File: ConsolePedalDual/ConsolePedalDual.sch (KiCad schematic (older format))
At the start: 20 parts, among them J1 AudioJack3, J2 AudioJack2, J3 Conn_02x25_Odd_Even, J4 Conn_02x25_Odd_Even, SW1 Bypass

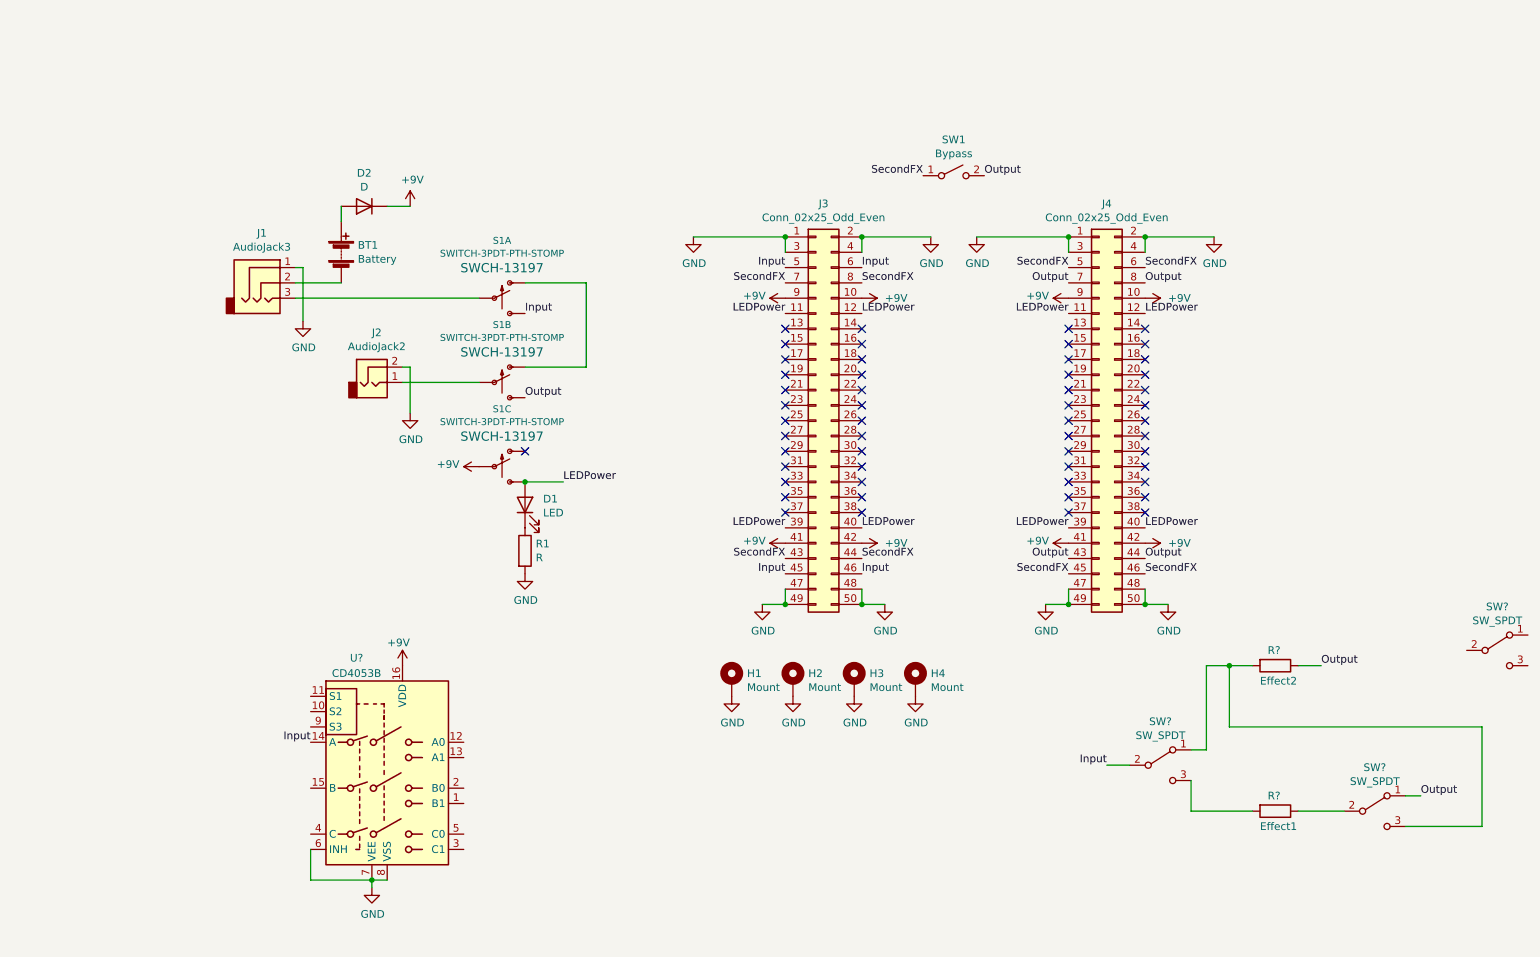
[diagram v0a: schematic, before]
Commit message: Finished schematic. Trying to figure out how to fit all these components on this board
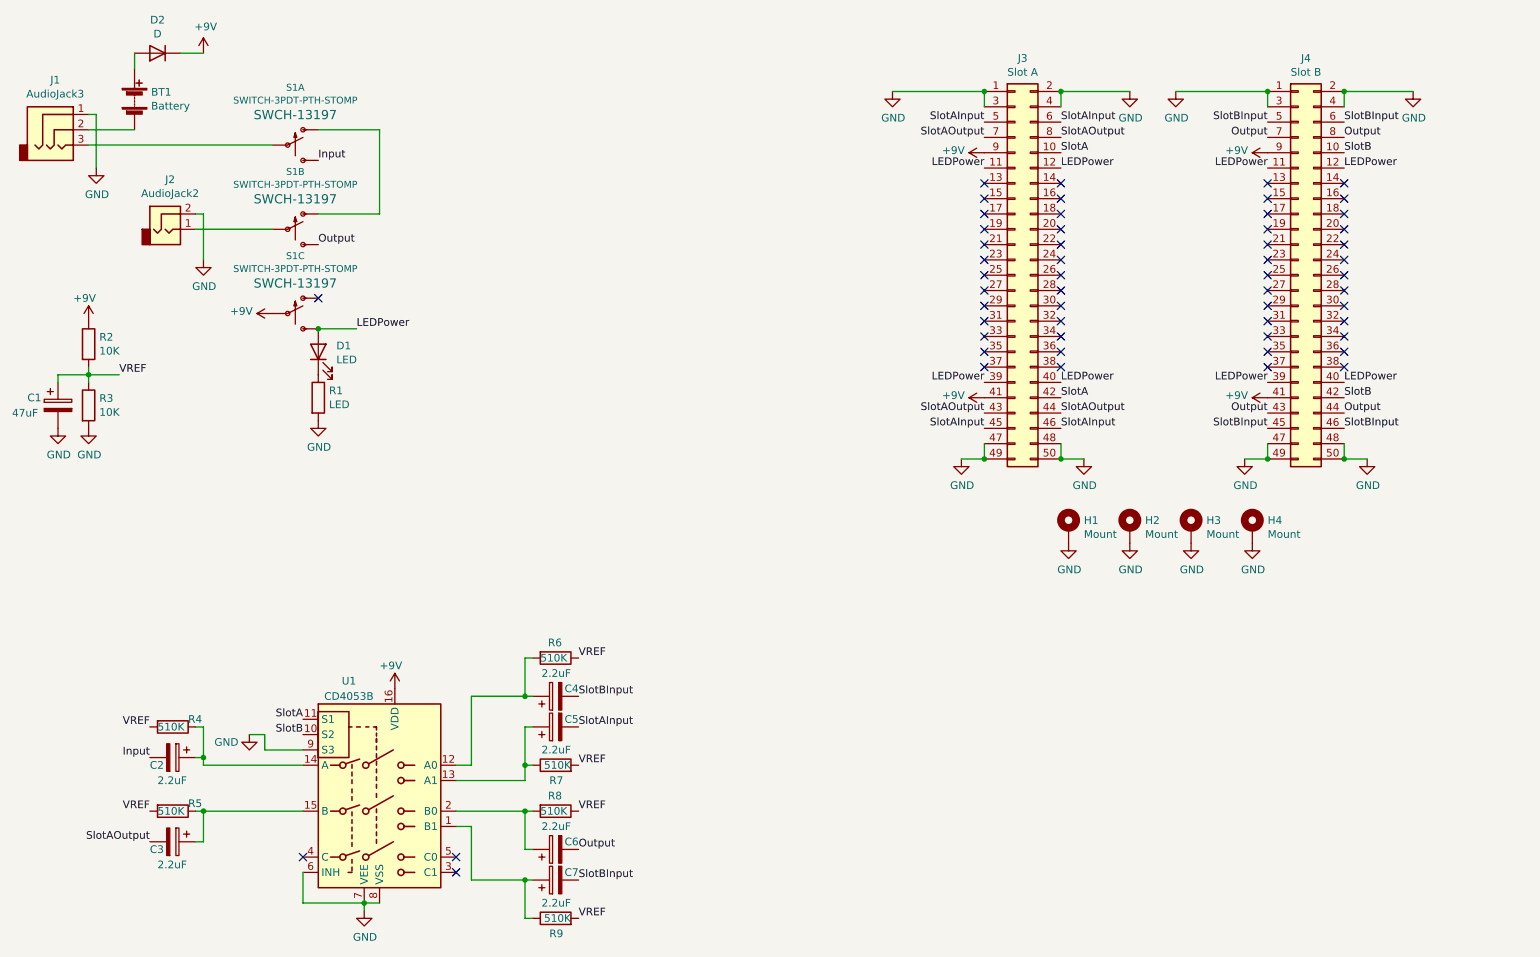
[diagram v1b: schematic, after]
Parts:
- removed R?: Effect1, Resistor_THT:R_Axial_DIN0207_L6.3mm_D2.5mm_P10.16mm_Horizontal, symbol Device:R
- removed R?: Effect2, Resistor_THT:R_Axial_DIN0207_L6.3mm_D2.5mm_P10.16mm_Horizontal, symbol Device:R
- removed SW1: Bypass, Connector_PinSocket_2.54mm:PinSocket_1x02_P2.54mm_Vertical, symbol Switch:SW_SPST
- removed SW? (x3): SW_SPDT, symbol Switch:SW_SPDT
- added C1: 47uF, Capacitor_THT:CP_Radial_D6.3mm_P2.50mm, symbol Device:CP
- added C2, C3, C4, C5, C6, C7: 2.2uF, Capacitor_THT:CP_Radial_D4.0mm_P2.00mm, symbol Device:CP
- added R2, R3: 10K, Resistor_THT:R_Axial_DIN0207_L6.3mm_D2.5mm_P10.16mm_Horizontal, symbol Device:R
- added R4, R5, R6, R7, R8, R9: 510K, Resistor_THT:R_Axial_DIN0207_L6.3mm_D2.5mm_P10.16mm_Horizontal, symbol Device:R
- J3: value Conn_02x25_Odd_Even -> Slot A
- J4: value Conn_02x25_Odd_Even -> Slot B
- R1: value R -> LED
- U1: renamed from U?; footprint (none) -> Package_DIP:DIP-16_W7.62mm_Socket
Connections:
- net +9V: now also R2.1; no longer J3.10 (Pin_10), J3.42 (Pin_42), J4.10 (Pin_10), J4.42 (Pin_42)
- net GND: now also U1.9 (S3), C1.2, R3.2
- net Input: now also C2.2; no longer J3.45 (Pin_45), J3.46 (Pin_46), J3.5 (Pin_5), J3.6 (Pin_6), U1.14 (A)
- net Output: now also C6.2
- net at U1.1 (B1): now also C7.1, R9.1
- net SlotB: now reaches U1.10 (S2)
- net SlotB: now also J4.10 (Pin_10), J4.42 (Pin_42)
- net SlotA: now reaches U1.11 (S1)
- net SlotA: now also J3.10 (Pin_10), J3.42 (Pin_42)
- net at U1.12 (A0): now also C4.1, R6.2
- net at U1.13 (A1): now also C5.1, R7.1
- net at U1.15 (B): now also C3.1, R5.1
- net at U1.2 (B0): now also C6.1, R8.2
- net SecondFX renamed SlotAOutput
- net SlotAOutput: now also C3.2; no longer J4.45 (Pin_45), J4.46 (Pin_46), J4.5 (Pin_5), J4.6 (Pin_6)
- new net: C2.1, R4.1, U1.14 (A)
- new net SlotAInput: C5.2, J3.45 (Pin_45), J3.46 (Pin_46), J3.5 (Pin_5), J3.6 (Pin_6)
- new net SlotBInput: C4.2, C7.2, J4.45 (Pin_45), J4.46 (Pin_46), J4.5 (Pin_5), J4.6 (Pin_6)
- new net VREF: C1.1, R2.2, R3.1, R4.2, R5.2, R6.1, R7.2, R8.1, R9.2
- no-connect marks 53 -> 56
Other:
- moved on the sheet: BT1, D1, D2, H1, H2, H3, H4, J1, J2, J3, J4, R1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
